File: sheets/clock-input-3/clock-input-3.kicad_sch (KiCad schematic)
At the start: 14 parts, among them U1 40106

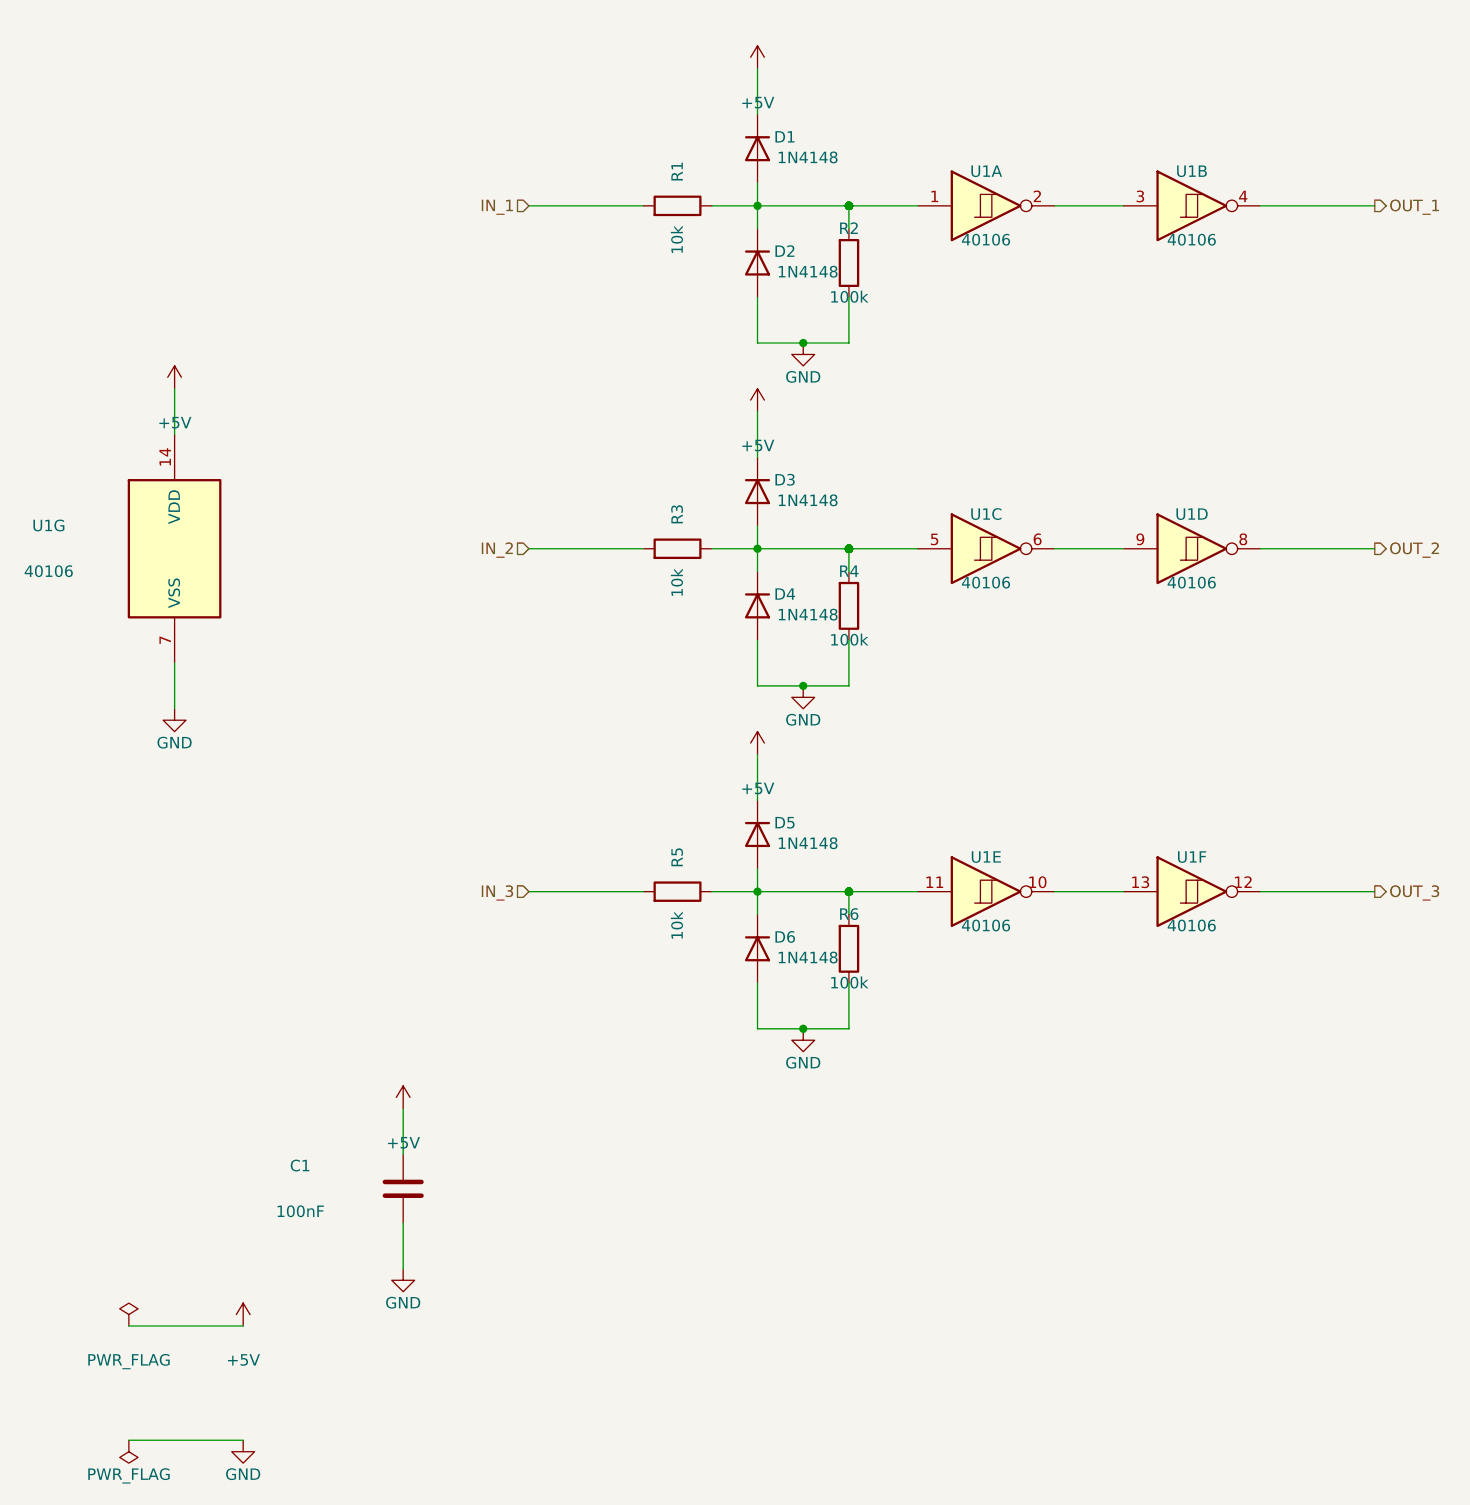
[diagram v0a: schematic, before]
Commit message: Record the missing root sheet instance
Co-Authored-By: Claude Opus 5 (1M context) <noreply@anthropic.com>
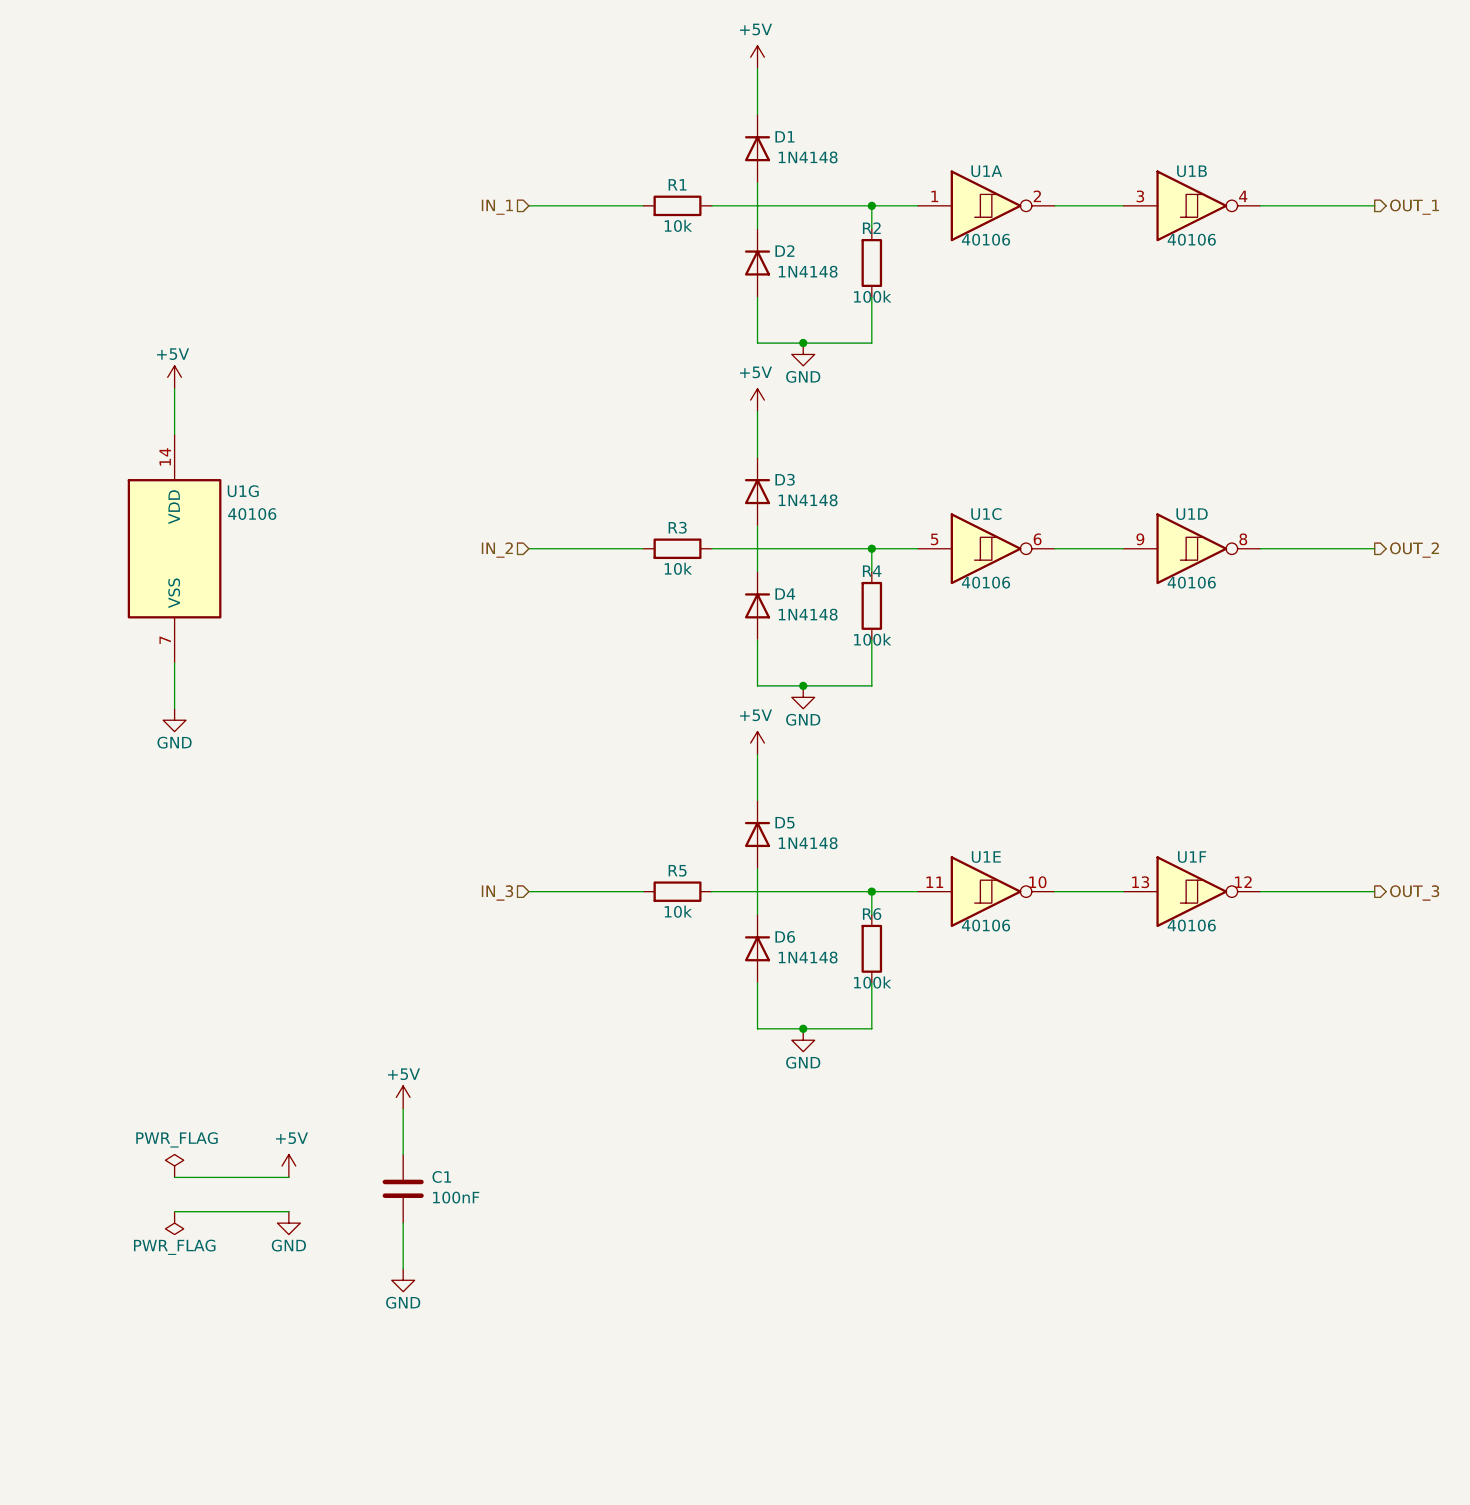
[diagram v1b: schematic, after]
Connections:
- net at R5.2, R6.1, U1.11: no longer D5.2 (A), D6.1 (K)
- net at R3.2, R4.1, U1.5: no longer D3.2 (A), D4.1 (K)
- net at R1.2, R2.1, U1.1: no longer D1.2 (A), D2.1 (K)
- new net: D1.2 (A), D2.1 (K)
- new net: D5.2 (A), D6.1 (K)
- new net: D3.2 (A), D4.1 (K)
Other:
- moved on the sheet: R2, R4, R6
